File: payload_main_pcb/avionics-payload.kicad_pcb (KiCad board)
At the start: 2 copper layers, 80 x 80 mm, 27 parts, among them J1 Micro_SD_Card, J2 Conn_Coaxial_x2, J3 Screw_Terminal_01x02, SW1 SW_Push, SW2 SW_Push, SW3 SW_Push, U2 Teensy4.0, U3 RFM96W-433S2, U4 LT1129-3.3_SOT223, U5 ublox_SAM-M8Q, U6 MS5607-02BA, U7 ADIS16470AMLZ

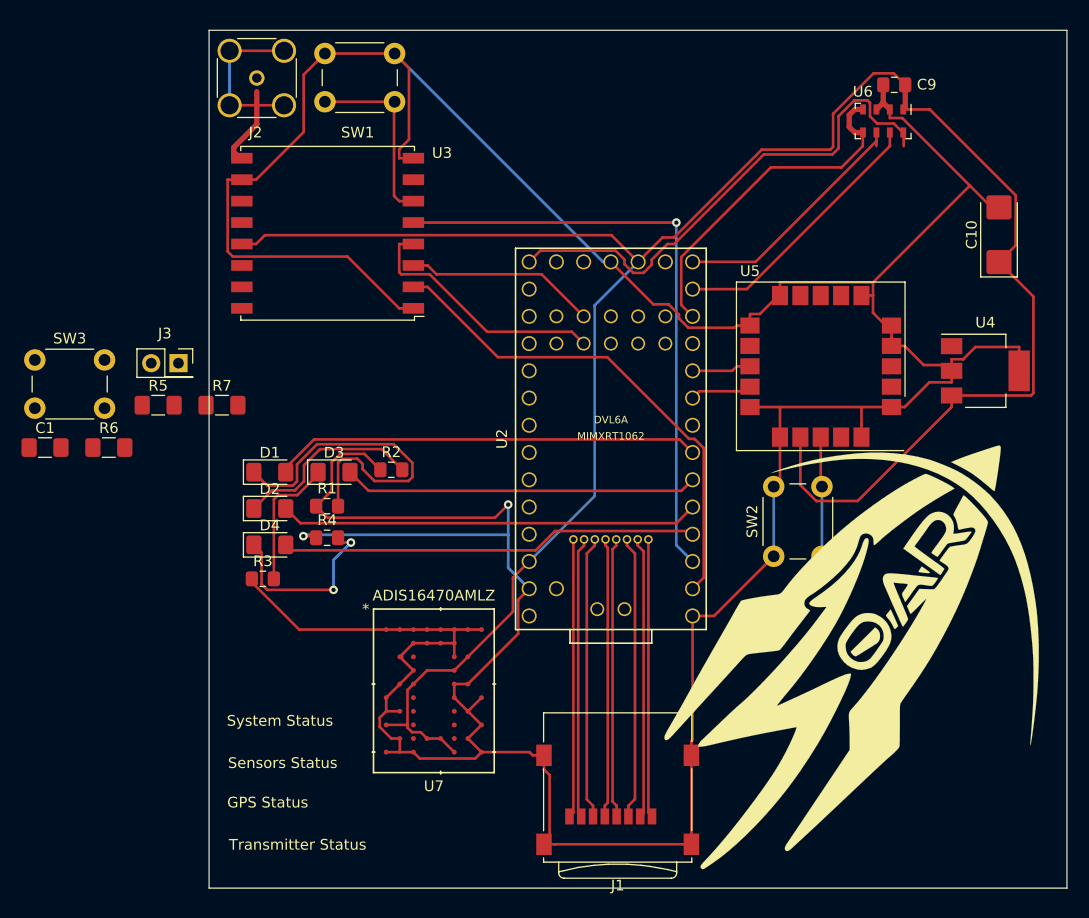
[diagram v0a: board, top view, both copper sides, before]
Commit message: Lots of stuff
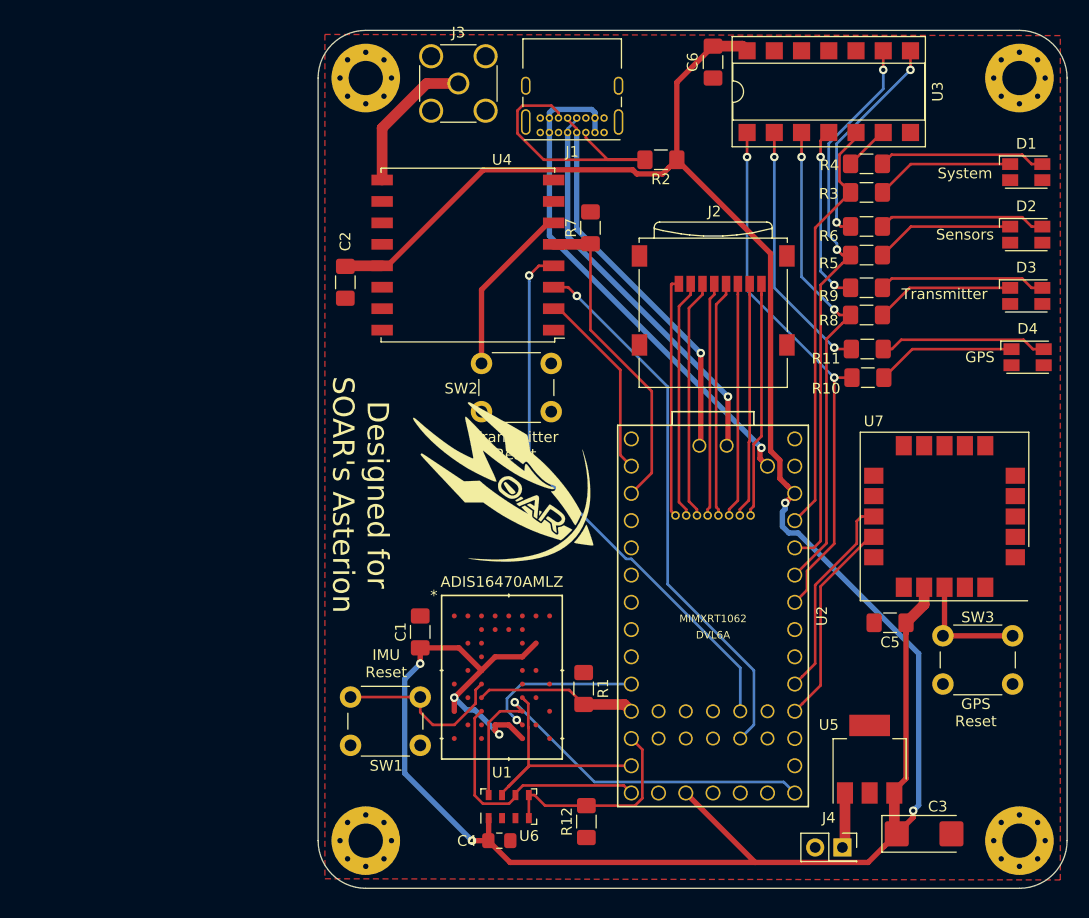
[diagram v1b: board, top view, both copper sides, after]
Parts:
- removed the J2 at (44.5, 44.5)
- removed the R1 at (51.0, 84.4)
- removed the Ref** at (69.8, 75.6)
- added C2: 100nF, Capacitor_SMD:C_1206_3216Metric_Pad1.42x1.75mm_HandSolder, F.Cu at (52.7, 63.5)
- added C5: 100nF, Capacitor_SMD:C_1206_3216Metric_Pad1.42x1.75mm_HandSolder, F.Cu at (103.5, 95.2)
- added C6: 100nF, Capacitor_SMD:C_1206_3216Metric_Pad1.42x1.75mm_HandSolder, F.Cu at (87.0, 43.0)
- added J1: USB_C_Receptacle_USB2.0, Connector_USB:USB_C_Receptacle_GCT_USB4085, F.Cu at (76.8, 49.5)
- added J3: Conn_Coaxial, Connector_Coaxial:SMA_Amphenol_132291_Vertical, F.Cu at (63.2, 45.0)
- added R10: 51, Resistor_SMD:R_1206_3216Metric_Pad1.42x1.75mm_HandSolder, F.Cu at (101.4, 72.4)
- added R11: 10, Resistor_SMD:R_1206_3216Metric_Pad1.42x1.75mm_HandSolder, F.Cu at (101.4, 69.7)
- added R5: 51, Resistor_SMD:R_1206_3216Metric_Pad1.42x1.75mm_HandSolder, F.Cu at (101.3, 61.0)
- added R6: 10, Resistor_SMD:R_1206_3216Metric_Pad1.42x1.75mm_HandSolder, F.Cu at (101.3, 58.3)
- added R8: 51, Resistor_SMD:R_1206_3216Metric_Pad1.42x1.75mm_HandSolder, F.Cu at (101.3, 66.5)
- added R9: 10, Resistor_SMD:R_1206_3216Metric_Pad1.42x1.75mm_HandSolder, F.Cu at (101.3, 64.0)
- added REF**: MountingHole_3.2mm_M3_Pad_Via, MountingHole:MountingHole_3.2mm_M3_Pad_Via, F.Cu at (54.6, 44.5)
- added REF**: MountingHole_3.2mm_M3_Pad_Via, MountingHole:MountingHole_3.2mm_M3_Pad_Via, F.Cu at (54.6, 115.6)
- added REF**: MountingHole_3.2mm_M3_Pad_Via, MountingHole:MountingHole_3.2mm_M3_Pad_Via, F.Cu at (115.6, 44.5)
- added REF**: MountingHole_3.2mm_M3_Pad_Via, MountingHole:MountingHole_3.2mm_M3_Pad_Via, F.Cu at (115.6, 115.6)
- added Ref**: Val**, footprints:logo, F.Cu at (36.3, 114.3)
- added U3: 74LS14, Package_DIP:DIP-14_W7.62mm_SMDSocket_SmallPads, F.Cu at (97.8, 45.7)
- D1, D2, D3, D4: value LED -> LED_RGBA; footprint LED_SMD:LED_1206_3216Metric_Pad1.42x1.75mm_HandSolder -> LED_SMD:LED_Avago_PLCC4_3.2x2.8mm_CW
- R2: value 220 -> R; footprint Resistor_SMD:R_0805_2012Metric_Pad1.15x1.40mm_HandSolder -> Resistor_SMD:R_1206_3216Metric_Pad1.42x1.75mm_HandSolder
- R3: value 220 -> 51; footprint Resistor_SMD:R_0805_2012Metric_Pad1.15x1.40mm_HandSolder -> Resistor_SMD:R_1206_3216Metric_Pad1.42x1.75mm_HandSolder
- R4: value 220 -> 10; footprint Resistor_SMD:R_0805_2012Metric_Pad1.15x1.40mm_HandSolder -> Resistor_SMD:R_1206_3216Metric_Pad1.42x1.75mm_HandSolder
- moved C4 79.5 mm to (67.1, 115.6), turned to 0 degrees
- moved J4 76.6 mm to (99.1, 116.2)
- moved D1 75.9 mm to (116.2, 53.2)
- moved D2 75.0 mm to (116.2, 59.1)
- moved U6 72.9 mm to (67.9, 112.4), turned to 90 degrees
- moved D4 72.8 mm to (116.3, 70.5)
- moved R3 66.8 mm to (101.3, 55.1), turned to 180 degrees
- moved D3 66.6 mm to (116.2, 64.8)
- moved R4 61.2 mm to (101.3, 52.5), turned to 180 degrees
- moved C3 56.3 mm to (106.7, 114.9), turned to 0 degrees
- moved R12 51.6 mm to (75.2, 113.8), turned to 90 degrees
- moved SW1 50.8 mm to (59.7, 106.7), turned to 180 degrees
- moved R7 49.4 mm to (75.6, 58.4), turned to 90 degrees
- moved R1 47.7 mm to (74.9, 101.4), turned to 270 degrees
- moved J2 47.4 mm to (87.0, 65.2), turned to 0 degrees
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- renumbered C10 to C3, C9 to C4, J1 to J2, J3 to J4, R5 to R1, R7 to R12, R6 to R7, SW3 to SW1, SW1 to SW2, SW2 to SW3, U7 to U1, U3 to U4, U4 to U5, U5 to U7
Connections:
- D1 pad 2: SystemStatus -> Net-(D1-Pad2)
- D2 pad 2: SensorStatus -> Net-(D2-Pad2)
- D3 pad 2: TransmitterStatus -> Net-(D3-Pad2)
- D4 pad 2: GPSStatus -> Net-(D4-Pad2)
- R2 pad 1: GND -> +3V3
- R2 pad 2: Net-(D2-Pad1) -> Net-(J1-PadA5)
- R3 pad 1: GND -> Net-(D1-Pad1)
- R3 pad 2: Net-(D3-Pad1) -> SystemStatus
- R4 pad 1: GND -> Net-(D1-Pad2)
- R4 pad 2: Net-(D4-Pad1) -> Net-(R4-Pad2)
- U2 pad 10: TX1 -> IMU_DR
- U2 pad 23: Net-(U2-Pad23) -> RX1
- U2 pad 24: Net-(U2-Pad24) -> TX1
- U2 pad 27: Net-(U2-Pad27) -> GPSStatus
- U2 pad 28: IMU_DR -> TransmitterStatus
- U2 pad 29: Net-(U2-Pad29) -> SensorStatus
- U2 pad 30: Net-(U2-Pad30) -> SystemStatus
- U2 pad 34: Net-(U2-Pad34) -> V_USB
- U2 pad 4: GPSStatus -> Net-(U2-Pad4)
- U2 pad 5: SensorStatus -> Net-(U2-Pad5)
- U2 pad 53: Net-(U2-Pad53) -> USB_D-
- U2 pad 54: Net-(U2-Pad54) -> USB_D+
- U2 pad 6: TransmitterStatus -> Net-(U2-Pad6)
- U2 pad 7: SystemStatus -> Net-(U2-Pad7)
- U2 pad 9: RX1 -> Net-(U2-Pad9)
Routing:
- net GND: track 408.1 -> 0.00 mm, vias 2 -> 0
- net +3V3: track 202.1 -> 251.5 mm, vias 0 -> 6
- net V_USB: track 0.00 -> 47.8 mm, vias 0 -> 1
- net USB_D-: track 0.00 -> 37.2 mm, vias 0 -> 1
- net USB_D+: track 0.00 -> 35.8 mm, vias 0 -> 1
- net MOSI2: track 17.8 -> 51.1 mm, vias 0 -> 1
- net MISO2: track 46.8 -> 18.0 mm
- net SCK2: track 23.9 -> 51.7 mm, vias 0 -> 1
- net CS2: track 56.8 -> 29.9 mm, vias 1 -> 0
- net Net-(J1-PadA5): track 0.00 -> 25.9 mm
- net Net-(R11-Pad2): track 0.00 -> 24.0 mm, vias 0 -> 2
- net Net-(R6-Pad2): track 0.00 -> 20.3 mm, vias 0 -> 2
- net Net-(D1-Pad1): track 32.3 -> 13.0 mm
- net Net-(R9-Pad2): track 0.00 -> 16.7 mm, vias 0 -> 2
- net Net-(SW1-Pad2): track 0.00 -> 16.4 mm
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- added copper zone on F.Cu, net GND
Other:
- board size 80 x 80 mm -> 69.8 x 80 mm
- board text added: "Designed for SOAR's Asterion"
- board text added: "GPS"
- board text added: "GPS Reset"
- board text added: "IMU Reset"
- board text added: "Sensors"
- board text added: "System"
- board text added: "Transmitter"
- board text added: "Transmitter Reset"
- board text removed: "GPS Status"
- board text removed: "Sensors Status"
- board text removed: "System Status"
- board text removed: "Transmitter Status"
